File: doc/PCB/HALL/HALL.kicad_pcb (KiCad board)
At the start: 2 copper layers, 161.7 x 105.8 mm, 91 parts, among them J1 Conn_01x05_Female, J10 CHIN+, J11 CHIN-, J12 Vcc, J13 CHOUT+, J14 CHOUT-, J2 Digit1, J3 Conn_01x05_Female, J4 Digit2, J5 Conn_01x05_Female, J6 Digit3, J7 Conn_01x05_Female, J8 Digit4, J9 PILOT, Q1 BC817-40, Q10 BC817-40, Q11 BC807-40, Q12 BC817-40, Q13 BC817-40, Q14 BC817-40, Q15 IRLR3636, Q16 BC817-40, Q2 BC807-40, Q3 BC817-40, Q4 BC817-40, Q5 BC807-40, Q6 BC817-40, Q7 BC817-40, Q8 BC807-40, Q9 BC817-40, SW1 UP, SW2 LEFT, SW3 RIGHT, SW4 DOWN, SW5 ENTER, SW6 BACK, U1 LM317_3PinPackage, U2 LM7812_TO220, U3 LM1117-3.3, U4 STM32F030K6Tx, U5 LM317_3PinPackage, Y1 Crystal

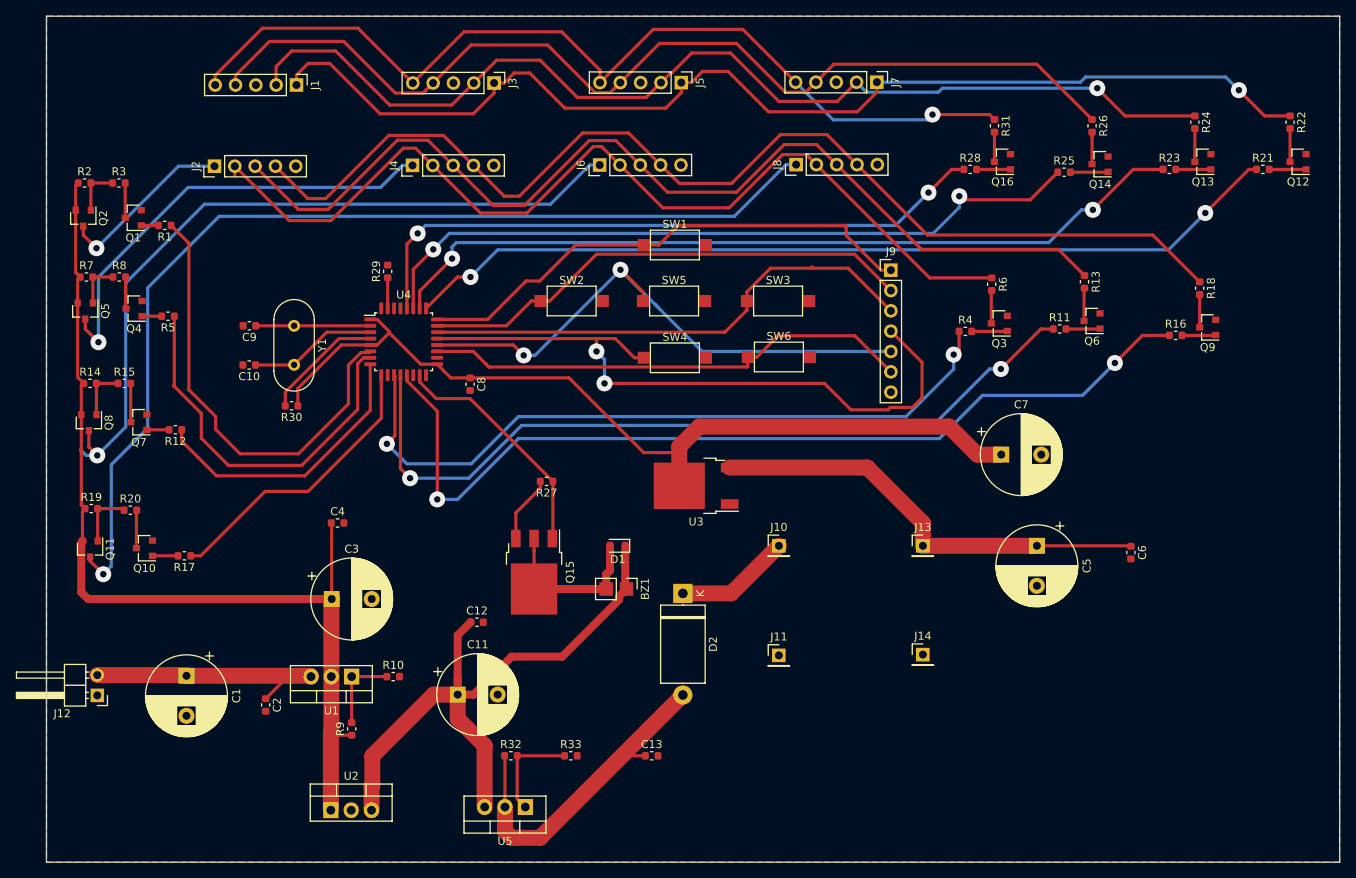
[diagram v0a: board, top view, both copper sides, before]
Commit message: new pcb
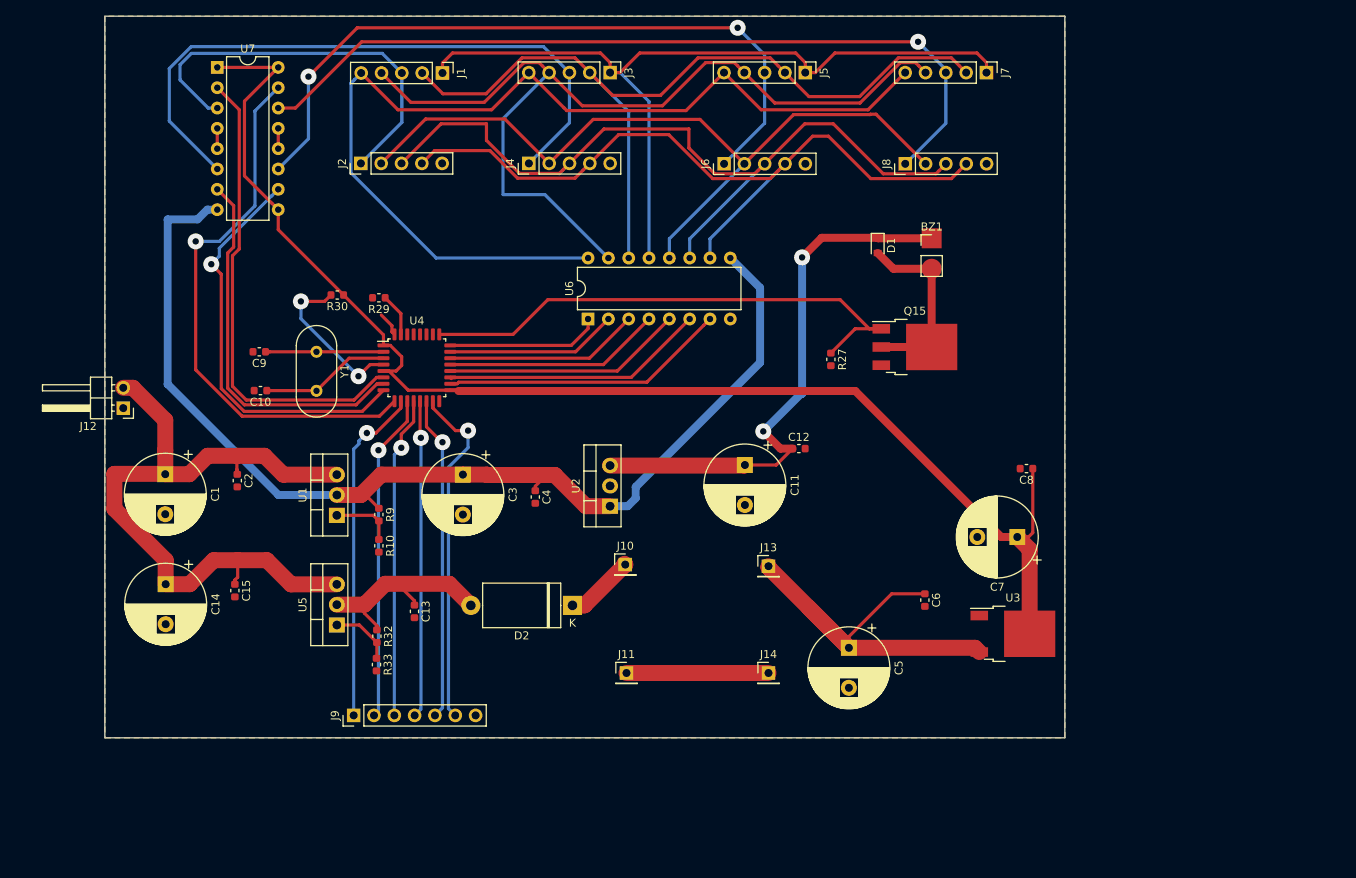
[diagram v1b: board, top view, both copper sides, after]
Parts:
- removed Q1, Q10, Q12, Q13, Q14, Q16, Q3, Q4, Q6, Q7, Q9: BC817-40, Package_TO_SOT_SMD:SOT-23
- removed Q11, Q2, Q5, Q8: BC807-40, Package_TO_SOT_SMD:SOT-23
- removed R1, R11, R12, R14, R16, R17, R19, R2, R21, R23, R25, R28, R4, R5, R7: 1k, Resistor_SMD:R_0603_1608Metric
- removed R13, R18, R22, R24, R26, R31, R6: 100R, Resistor_SMD:R_0603_1608Metric
- removed R15, R20, R3, R8: 10k, Resistor_SMD:R_0603_1608Metric
- removed SW1: UP, Button_Switch_SMD:SW_SPST_CK_RS282G05A3
- removed SW2: LEFT, Button_Switch_SMD:SW_SPST_CK_RS282G05A3
- removed SW3: RIGHT, Button_Switch_SMD:SW_SPST_CK_RS282G05A3
- removed SW4: DOWN, Button_Switch_SMD:SW_SPST_CK_RS282G05A3
- removed SW5: ENTER, Button_Switch_SMD:SW_SPST_CK_RS282G05A3
- removed SW6: BACK, Button_Switch_SMD:SW_SPST_CK_RS282G05A3
- added C14: 10u, Capacitor_THT:CP_Radial_D10.0mm_P5.00mm, F.Cu at (39.8, 83.0)
- added C15: 100n, Capacitor_SMD:C_0603_1608Metric, F.Cu at (48.5, 83.8)
- added U6: ULN2003, Package_DIP:DIP-16_W7.62mm, F.Cu at (92.6, 49.9)
- added U7: L293D, Package_DIP:DIP-16_W7.62mm, F.Cu at (46.2, 18.4)
- moved J9 87.2 mm to (63.3, 99.4), turned to 90 degrees
- moved C8 70.3 mm to (147.4, 68.5), turned to 180 degrees
- moved BZ1 57.4 mm to (135.6, 40.6), turned to 0 degrees
- moved Q15 55.3 mm to (133.4, 53.4), turned to 0 degrees
- moved U2 51.6 mm to (95.3, 73.2), turned to 90 degrees
- moved D1 49.7 mm to (128.8, 40.6), turned to 270 degrees
- moved C11 46.0 mm to (112.2, 68.1), turned to 270 degrees
- moved C12 45.7 mm to (119.0, 66.0)
- moved U3 43.7 mm to (145.7, 89.2), turned to 0 degrees
- moved R27 38.7 mm to (123.0, 54.9), turned to 270 degrees
- moved J12 36.1 mm to (34.5, 61.0)
- moved C13 34.7 mm to (70.9, 86.4), turned to 270 degrees
- moved U5 32.7 mm to (61.2, 88.1), turned to 90 degrees
- moved C2 28.3 mm to (48.8, 70.0)
- moved R9 27.0 mm to (66.5, 74.3), turned to 270 degrees
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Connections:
- J2 pad 1: Net-(J2-Pad1) -> Net-(J1-Pad3)
- J4 pad 1: Net-(J4-Pad1) -> Net-(J3-Pad3)
- J6 pad 1: Net-(J6-Pad1) -> Net-(J5-Pad3)
- J8 pad 1: Net-(J8-Pad1) -> Net-(J7-Pad3)
- J9 pad 3: BUTTON_RIGHT -> BUTTON_ENTER
- J9 pad 4: BUTTON_DOWN -> BUTTON_RIGHT
- J9 pad 5: BUTTON_ENTER -> BUTTON_DOWN
- U4 pad 10: Net-(U4-Pad10) -> BUTTON_UP
- U4 pad 11: SE -> BUTTON_LEFT
- U4 pad 12: SD -> BUTTON_ENTER
- U4 pad 13: SC -> BUTTON_RIGHT
- U4 pad 14: SP -> BUTTON_DOWN
- U4 pad 15: BELL -> BUTTON_BACK
- U4 pad 18: Net-(U4-Pad18) -> SC
- U4 pad 19: BUTTON_BACK -> SD
- U4 pad 20: BUTTON_ENTER -> SE
- U4 pad 21: BUTTON_DOWN -> SB
- U4 pad 22: BUTTON_RIGHT -> SA
- U4 pad 23: BUTTON_LEFT -> SF
- U4 pad 24: BUTTON_UP -> SG
- U4 pad 25: SB -> BELL
- U4 pad 26: SA -> SP
- U4 pad 27: SF -> Net-(U4-Pad27)
- U4 pad 28: SG -> Net-(U4-Pad28)
- U5 pad 3: +12V -> +24V
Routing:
- net Net-(J8-Pad1): track 128.4 -> 0.00 mm, vias 1 -> 0
- net Net-(J7-Pad3): track 0.00 -> 102.2 mm, vias 0 -> 1
- net Net-(J6-Pad1): track 94.3 -> 0.00 mm, vias 1 -> 0
- net Net-(J5-Pad3): track 0.00 -> 89.8 mm, vias 0 -> 2
- net SB: track 111.0 -> 27.2 mm, vias 2 -> 0
- net SC: track 117.1 -> 35.8 mm, vias 2 -> 0
- net Net-(J3-Pad3): track 0.00 -> 81.0 mm
- net SA: track 102.2 -> 24.3 mm, vias 2 -> 0
- net SF: track 91.7 -> 21.5 mm, vias 2 -> 0
- net SD: track 101.5 -> 33.2 mm, vias 2 -> 0
- net SG: track 81.5 -> 19.3 mm, vias 2 -> 0
- net SE: track 90.8 -> 30.1 mm, vias 2 -> 0
- net Net-(J4-Pad1): track 59.1 -> 0.00 mm, vias 1 -> 0
- net +24V: track 33.6 -> 89.3 mm
- net +3V3: track 114.4 -> 168.8 mm
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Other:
- board size 161.7 x 105.8 mm -> 120 x 90.2 mm
